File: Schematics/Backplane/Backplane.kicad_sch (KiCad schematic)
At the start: 21 parts, among them J1 Edge Connector (SLOT 1), J2 Edge Connector (SLOT 2), J3 Edge Connector (SLOT 3), J4 Edge Connector (SLOT 4), J5 Edge Connector (SLOT 5), J6 Conn_01x06_Socket

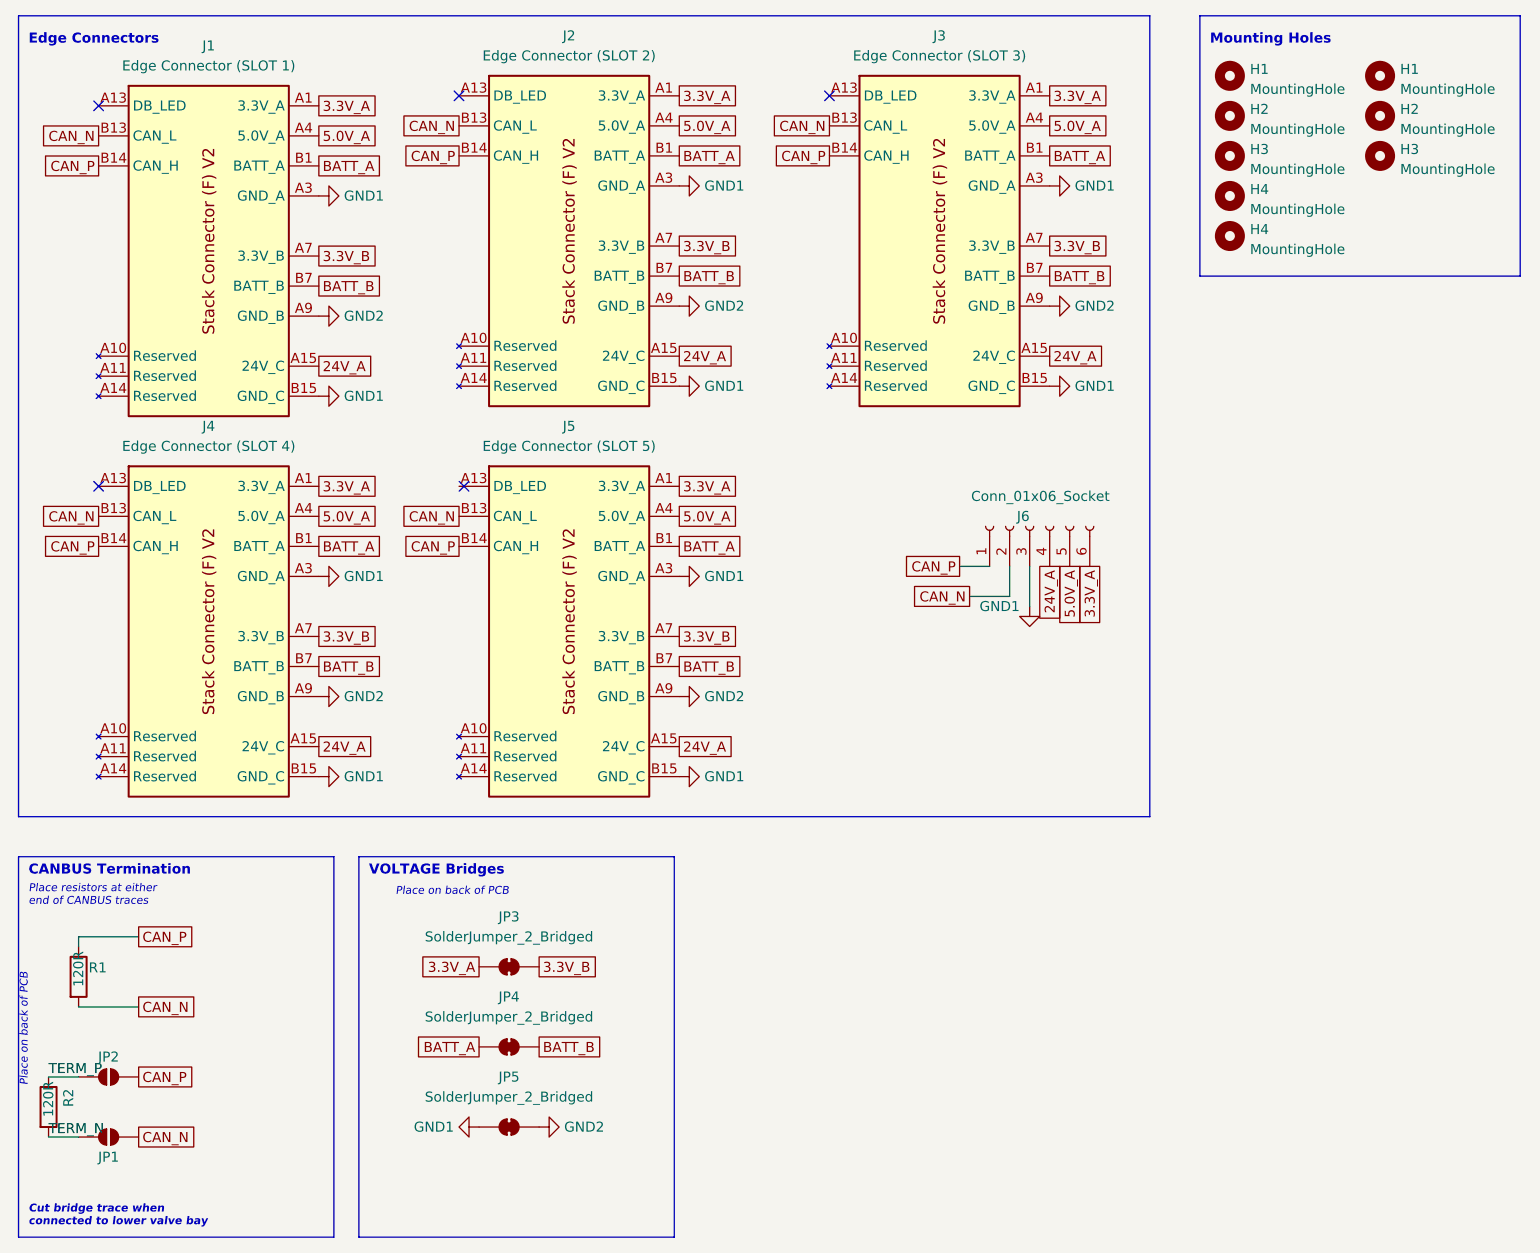
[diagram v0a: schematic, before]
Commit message: start of my own backplane layout
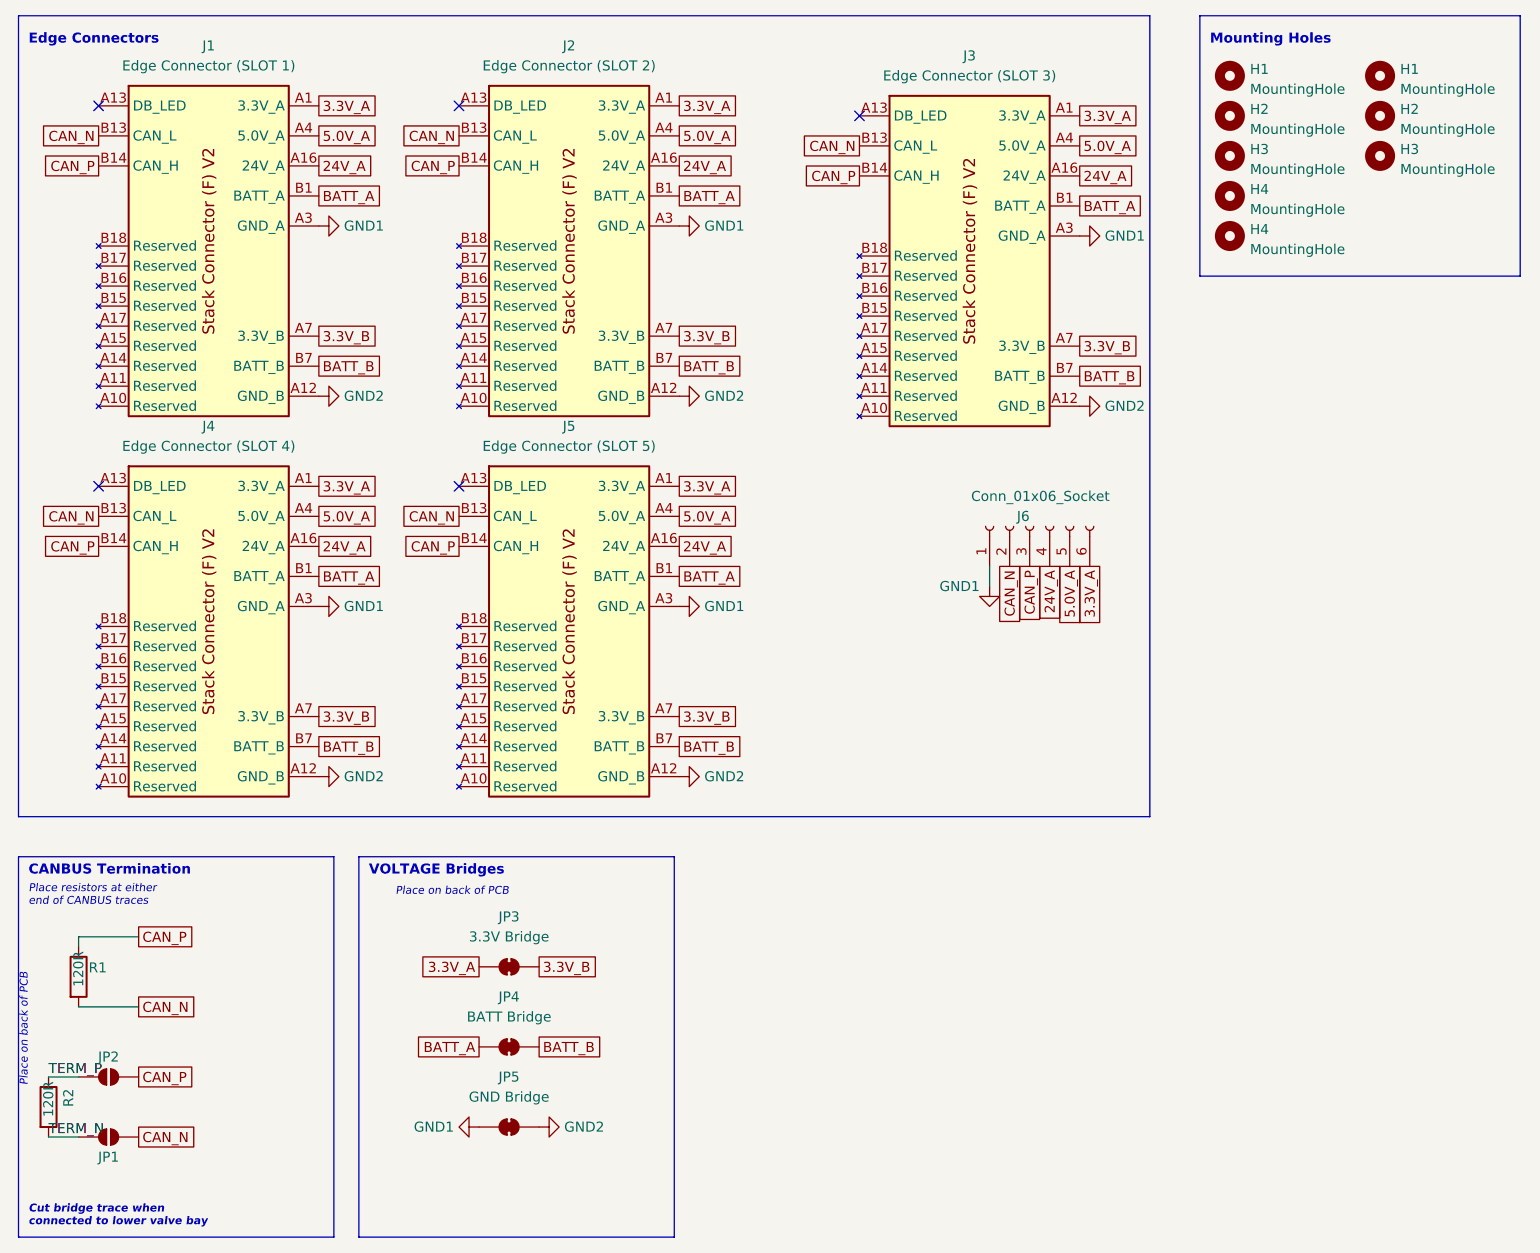
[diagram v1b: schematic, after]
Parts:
- removed J1: Edge Connector (SLOT 1), footprints:AMPHENOL_10018784-10210TLF, symbol EdgeConnnectorV1.1:Stack Female Edge Connector
- removed J2: Edge Connector (SLOT 2), footprints:AMPHENOL_10018784-10210TLF, symbol EdgeConnnectorV1.1:Stack Female Edge Connector
- removed J3: Edge Connector (SLOT 3), footprints:AMPHENOL_10018784-10210TLF, symbol EdgeConnnectorV1.1:Stack Female Edge Connector
- removed J4: Edge Connector (SLOT 4), footprints:AMPHENOL_10018784-10210TLF, symbol EdgeConnnectorV1.1:Stack Female Edge Connector
- removed J5: Edge Connector (SLOT 5), footprints:AMPHENOL_10018784-10210TLF, symbol EdgeConnnectorV1.1:Stack Female Edge Connector
- added J1: Edge Connector (SLOT 1), footprints:AMPHENOL_10018784-10210TLF, symbol EdgeConnnectorV2:Stack Female Edge Connector
- added J2: Edge Connector (SLOT 2), footprints:AMPHENOL_10018784-10210TLF, symbol EdgeConnnectorV2:Stack Female Edge Connector
- added J3: Edge Connector (SLOT 3), footprints:AMPHENOL_10018784-10210TLF, symbol EdgeConnnectorV2:Stack Female Edge Connector
- added J4: Edge Connector (SLOT 4), footprints:AMPHENOL_10018784-10210TLF, symbol EdgeConnnectorV2:Stack Female Edge Connector
- added J5: Edge Connector (SLOT 5), footprints:AMPHENOL_10018784-10210TLF, symbol EdgeConnnectorV2:Stack Female Edge Connector
- JP3: value SolderJumper_2_Bridged -> 3.3V Bridge
- JP4: value SolderJumper_2_Bridged -> BATT Bridge
- JP5: value SolderJumper_2_Bridged -> GND Bridge
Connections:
- net 24V_A: now also J1.A16 (24V_A), J1.A18 (24V_A), J2.A16 (24V_A), J2.A18 (24V_A), J3.A16 (24V_A), J3.A18 (24V_A), J4.A16 (24V_A), J4.A18 (24V_A), J5.A16 (24V_A), J5.A18 (24V_A)
- net 3.3V_A: now also J1.A1 (3.3V_A), J1.A2 (3.3V_A), J2.A1 (3.3V_A), J2.A2 (3.3V_A), J3.A1 (3.3V_A), J3.A2 (3.3V_A), J4.A1 (3.3V_A), J4.A2 (3.3V_A), J5.A1 (3.3V_A), J5.A2 (3.3V_A)
- net 3.3V_B: now also J1.A7 (3.3V_B), J1.A8 (3.3V_B), J2.A7 (3.3V_B), J2.A8 (3.3V_B), J3.A7 (3.3V_B), J3.A8 (3.3V_B), J4.A7 (3.3V_B), J4.A8 (3.3V_B), J5.A7 (3.3V_B), J5.A8 (3.3V_B)
- net 5.0V_A: now also J1.A4 (5.0V_A), J1.A5 (5.0V_A), J2.A4 (5.0V_A), J2.A5 (5.0V_A), J3.A4 (5.0V_A), J3.A5 (5.0V_A), J4.A4 (5.0V_A), J4.A5 (5.0V_A), J5.A4 (5.0V_A), J5.A5 (5.0V_A)
- net BATT_A: now also J1.B1 (BATT_A), J1.B2 (BATT_A), J1.B3 (BATT_A), J2.B1 (BATT_A), J2.B2 (BATT_A), J2.B3 (BATT_A), J3.B1 (BATT_A), J3.B2 (BATT_A), J3.B3 (BATT_A), J4.B1 (BATT_A), J4.B2 (BATT_A), J4.B3 (BATT_A), J5.B1 (BATT_A), J5.B2 (BATT_A), J5.B3 (BATT_A)
- net BATT_B: now also J1.B7 (BATT_B), J1.B8 (BATT_B), J1.B9 (BATT_B), J2.B7 (BATT_B), J2.B8 (BATT_B), J2.B9 (BATT_B), J3.B7 (BATT_B), J3.B8 (BATT_B), J3.B9 (BATT_B), J4.B7 (BATT_B), J4.B8 (BATT_B), J4.B9 (BATT_B), J5.B7 (BATT_B), J5.B8 (BATT_B), J5.B9 (BATT_B)
- net CAN_N: now also J1.B13 (CAN_L), J2.B13 (CAN_L), J3.B13 (CAN_L), J4.B13 (CAN_L), J5.B13 (CAN_L)
- net CAN_P: now also J6.3 (Pin_3), J1.B14 (CAN_H), J2.B14 (CAN_H), J3.B14 (CAN_H), J4.B14 (CAN_H), J5.B14 (CAN_H); no longer J6.1 (Pin_1)
- net GND1: now also J6.1 (Pin_1), J1.A3 (GND_A), J1.A6 (GND_A), J1.B4 (GND_A), J1.B5 (GND_A), J1.B6 (GND_A), J2.A3 (GND_A), J2.A6 (GND_A), J2.B4 (GND_A), J2.B5 (GND_A), J2.B6 (GND_A), J3.A3 (GND_A), J3.A6 (GND_A), J3.B4 (GND_A), J3.B5 (GND_A), J3.B6 (GND_A), J4.A3 (GND_A), J4.A6 (GND_A), J4.B4 (GND_A), J4.B5 (GND_A), J4.B6 (GND_A), J5.A3 (GND_A), J5.A6 (GND_A), J5.B4 (GND_A), J5.B5 (GND_A), J5.B6 (GND_A); no longer J6.3 (Pin_3)
- net GND2: now also J1.A12 (GND_B), J1.A9 (GND_B), J1.B10 (GND_B), J1.B11 (GND_B), J1.B12 (GND_B), J2.A12 (GND_B), J2.A9 (GND_B), J2.B10 (GND_B), J2.B11 (GND_B), J2.B12 (GND_B), J3.A12 (GND_B), J3.A9 (GND_B), J3.B10 (GND_B), J3.B11 (GND_B), J3.B12 (GND_B), J4.A12 (GND_B), J4.A9 (GND_B), J4.B10 (GND_B), J4.B11 (GND_B), J4.B12 (GND_B), J5.A12 (GND_B), J5.A9 (GND_B), J5.B10 (GND_B), J5.B11 (GND_B), J5.B12 (GND_B)
